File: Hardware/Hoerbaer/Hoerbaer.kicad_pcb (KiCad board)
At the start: 4 copper layers, 80 x 88 mm, 198 parts, among them J1 I2C, J12 Battery 1S Li-Ion, J13 JTAG, J14 Speaker_L, J15 Speaker_R, J16 USB2_UART, J17 RST_BOOT, J2 DISPLAY, J3 Micro_SD_Card_Det1, J4 USB1, J5 ENCODER, J6 PAW_A, J7 PAW_B, J8 PAW_C, J9 PAW_D, Q1 DMG3415UQ-7, Q5 S8050, Q6 S8050, SW1 RESET, SW2 PROG, U1 ESP32 S3 MINI, U10 TAS5805M, U11 CH343P, U12 MAX17048G, U13 TPS61288, U2 PCF8574APWR, U3 PCF8574APWR, U4 PCF8574APWR, U5 TLC59108xPW, U6 TLC59108xPW, U7 TLC59108xPW, U8 MCP73831T-2ACI/OT (4.2V), U9 TPS63001

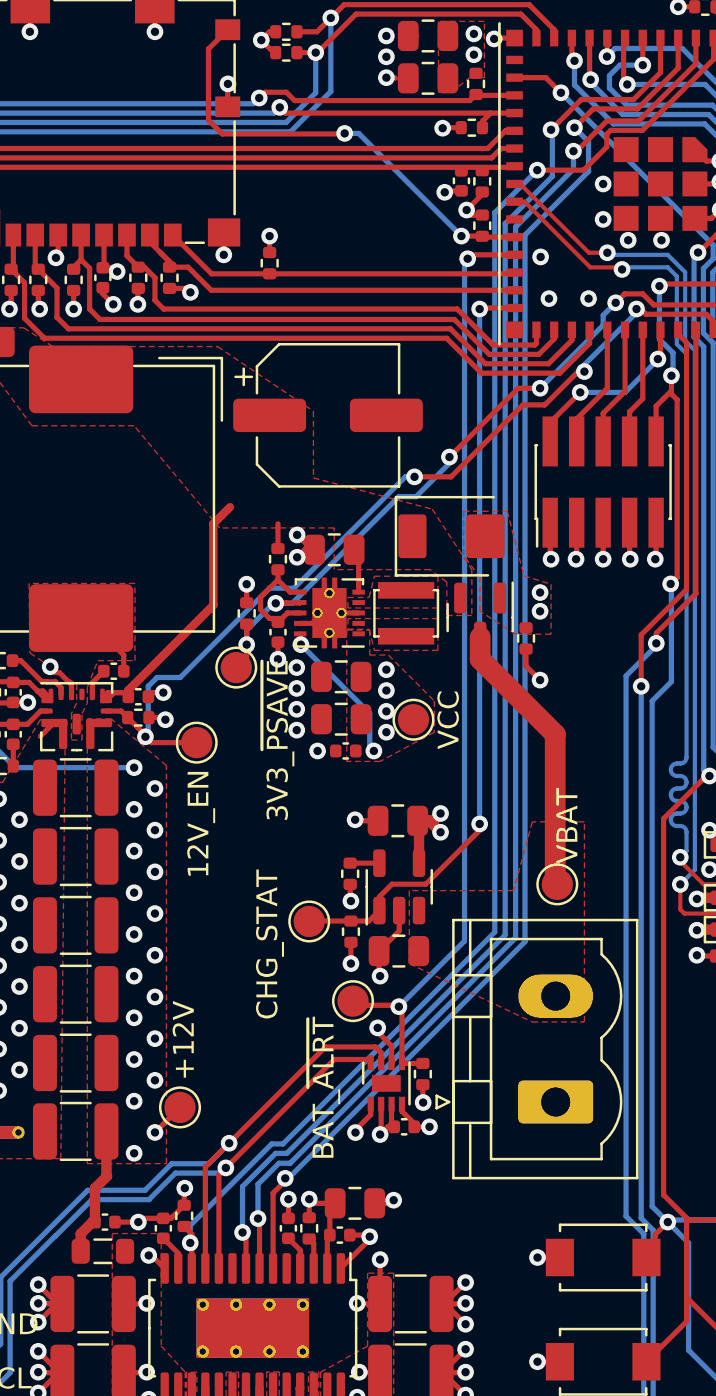
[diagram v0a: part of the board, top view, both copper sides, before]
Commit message: Order numbers
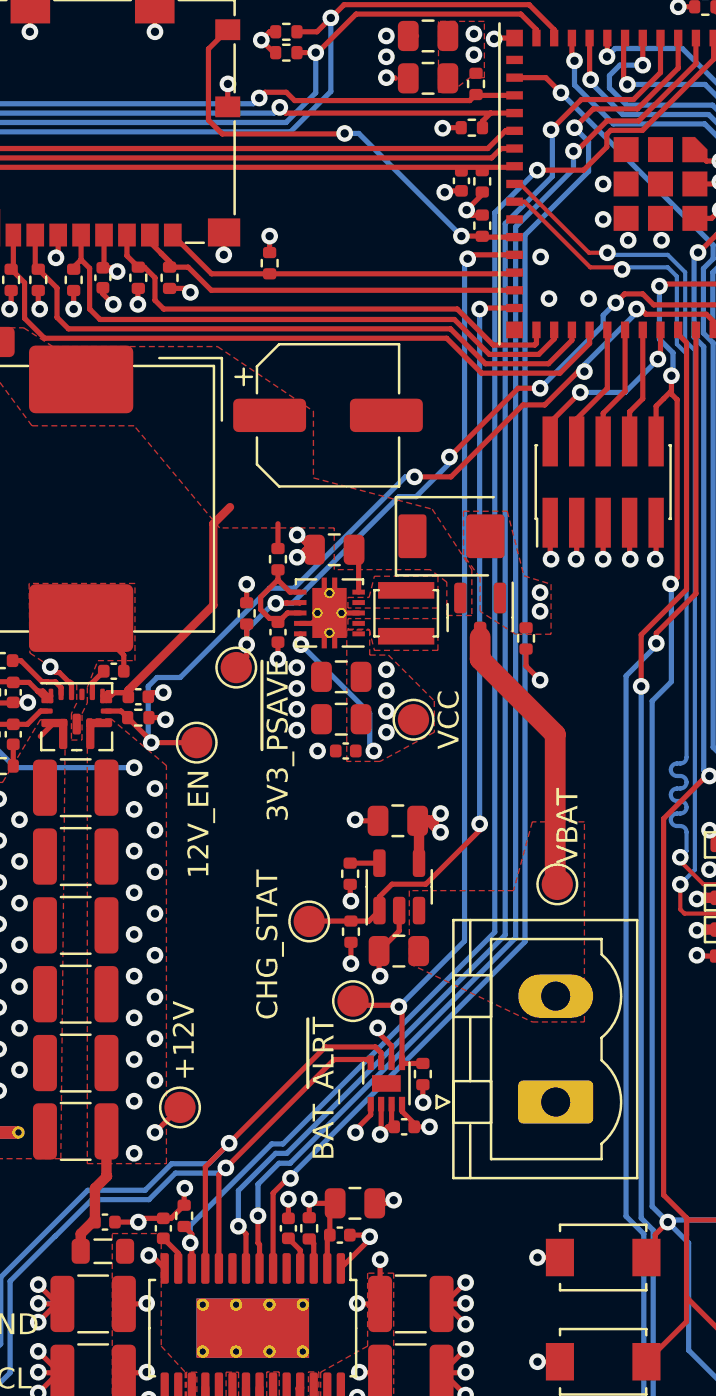
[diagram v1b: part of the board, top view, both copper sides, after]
